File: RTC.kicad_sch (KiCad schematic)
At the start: 10 parts, among them U5 PCF8563TS, Y2 MC-306

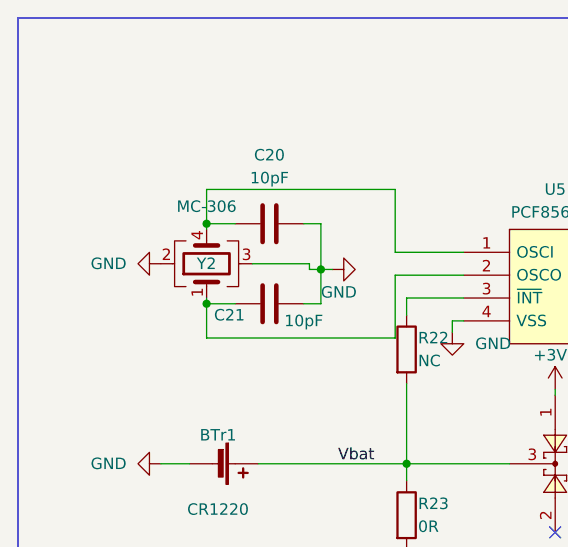
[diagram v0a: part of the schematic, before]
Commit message: Feat: Components's layout
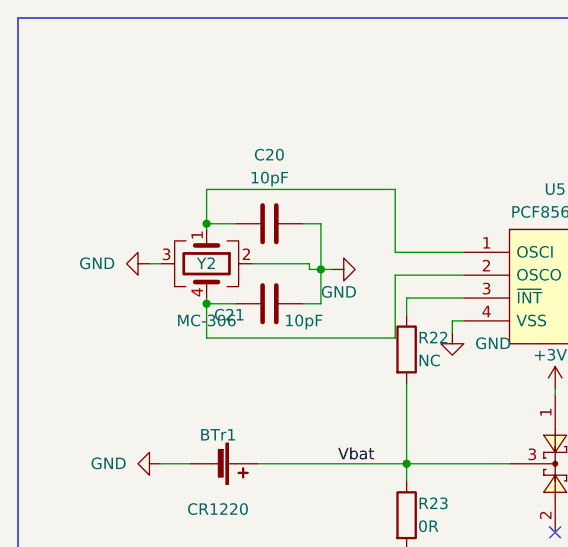
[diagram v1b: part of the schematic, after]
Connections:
- net at C21.1, U5.2 (OSCO): now also Y2.4; no longer Y2.1
- net at C20.1, U5.1 (OSCI): now also Y2.1; no longer Y2.4
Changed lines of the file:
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@@
+	(wire
+		(pts
+			(xy 51.435 51.435) (xy 52.705 51.435)
+		)
+		(stroke
+			(width 0)
+			(type default)
+		)
+	)
 	(wire
 		(pts
@@
 	(symbol
 		(lib_id "power:GND")
-		(at 52.705 51.435 270)
+		(at 51.435 51.435 270)
 		(unit 1)
 		(exclude_from_sim no)
@@
 		(fields_autoplaced yes)
 		(property "Reference" "#PWR031"
-			(at 46.355 51.435 0)
+			(at 45.085 51.435 0)
 			(effects
 				(font
@@
 		)
 		(property "Value" "GND"
-			(at 48.895 51.4349 90)
+			(at 47.625 51.4349 90)
 			(effects
 				(font
@@
 		)
 		(property "Footprint" ""
-			(at 52.705 51.435 0)
+			(at 51.435 51.435 0)
 			(effects
 				(font
@@
 		)
 		(property "Datasheet" ""
-			(at 52.705 51.435 0)
+			(at 51.435 51.435 0)
 			(effects
 				(font
@@
 		)
 		(property "Description" ""
-			(at 52.705 51.435 0)
+			(at 51.435 51.435 0)
 			(effects
 				(font
@@
 	)
 	(symbol
+		(lib_id "Device:Crystal_GND23")
+		(at 57.785 51.435 270)
+		(unit 1)
+		(exclude_from_sim no)
+		(in_bom yes)
+		(on_board yes)
+		(dnp no)
+		(property "Reference" "Y2"
+			(at 57.785 51.435 90)
+			(effects
+				(font
+					(size 1.27 1.27)
+				)
+			)
+		)
+		(property "Value" "MC-306"
+			(at 57.785 57.785 90)
+			(effects
+				(font
+					(size 1.27 1.27)
+				)
+			)
+		)
+		(property "Footprint" "Crystal:Crystal_SMD_SeikoEpson_MC306-4Pin_8.0x3.2mm"
+			(at 57.785 51.435 0)
+			(effects
+				(font
+					(size 1.27 1.27)
+				)
+				(hide yes)
+			)
+		)
+		(property "Datasheet" "~"
+			(at 57.785 51.435 0)
+			(effects
+				(font
+					(size 1.27 1.27)
+				)
+				(hide yes)
+			)
+		)
+		(property "Description" ""
+			(at 57.785 51.435 0)
+			(effects
+				(font
+					(size 1.27 1.27)
+				)
+				(hide yes)
+			)
+		)
+		(pin "1"
+		)
+		(pin "2"
+		)
+		(pin "3"
+		)
+		(pin "4"
+		)
+		(instances
+			(project "DongTamV2"
+				(path "/2303d546-b88a-4ab0-aee1-26e3b32ac9d7/4db09d46-189e-4d6b-adc1-7214f7292c64"
+					(reference "Y2")
+					(unit 1)
+				)
+			)
+		)
+	)
+	(symbol
 		(lib_id "Device:R")
 		(at 80.01 79.375 0)
@@
 					(unit 1)
 				)
-			)
-		)
-	)
-	(symbol
-		(lib_id "Device:Crystal_GND23")
-		(at 57.785 51.435 90)
-		(unit 1)
-		(exclude_from_sim no)
-		(in_bom yes)
-		(on_board yes)
-		(dnp no)
-		(property "Reference" "Y2"
-			(at 57.785 51.435 90)
-			(effects
-				(font
-					(size 1.27 1.27)
-				)
-			)
-		)
-		(property "Value" "MC-306"
-			(at 57.785 45.085 90)
-			(effects
-				(font
-					(size 1.27 1.27)
-				)
-			)
-		)
-		(property "Footprint" "Crystal:Crystal_SMD_SeikoEpson_MC306-4Pin_8.0x3.2mm"
-			(at 57.785 51.435 0)
-			(effects
-				(font
-					(size 1.27 1.27)
-				)
-				(hide yes)
-			)
-		)
-		(property "Datasheet" "~"
-			(at 57.785 51.435 0)
-			(effects
-				(font
-					(size 1.27 1.27)
-				)
-				(hide yes)
-			)
-		)
-		(property "Description" ""
-			(at 57.785 51.435 0)
-			(effects
-				(font
-					(size 1.27 1.27)
-				)
-				(hide yes)
-			)
-		)
-		(pin "1"
-		)
-		(pin "2"
-		)
-		(pin "3"
-		)
-		(pin "4"
-		)
-		(instances
-			(project "DongTamV2"
-				(path "/2303d546-b88a-4ab0-aee1-26e3b32ac9d7/4db09d46-189e-4d6b-adc1-7214f7292c64"
-					(reference "Y2")
-					(unit 1)
-				)
-			)
-			(project "dongtam"
-				(path "/6833aec4-3d1d-4261-9b3e-f0452b565dd3/a9a99304-d65b-4ed1-854e-7f464f20419d"
-					(reference "Y?")
-					(unit 1)
-				)

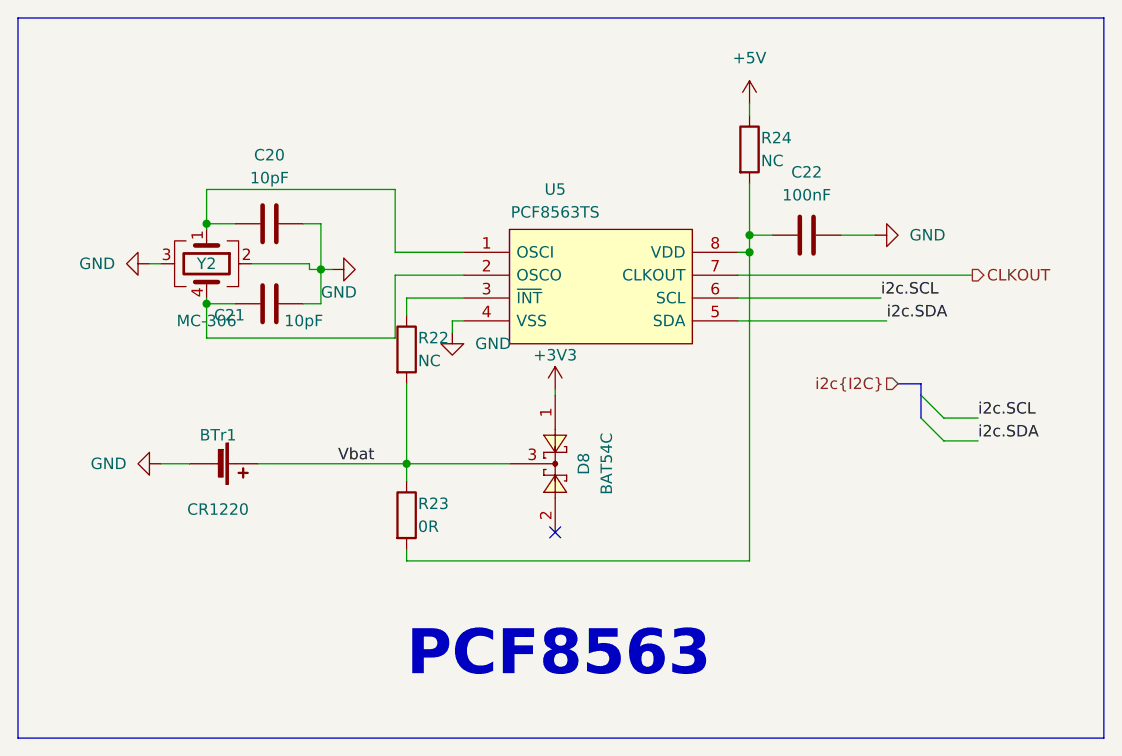
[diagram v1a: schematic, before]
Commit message: layout p1
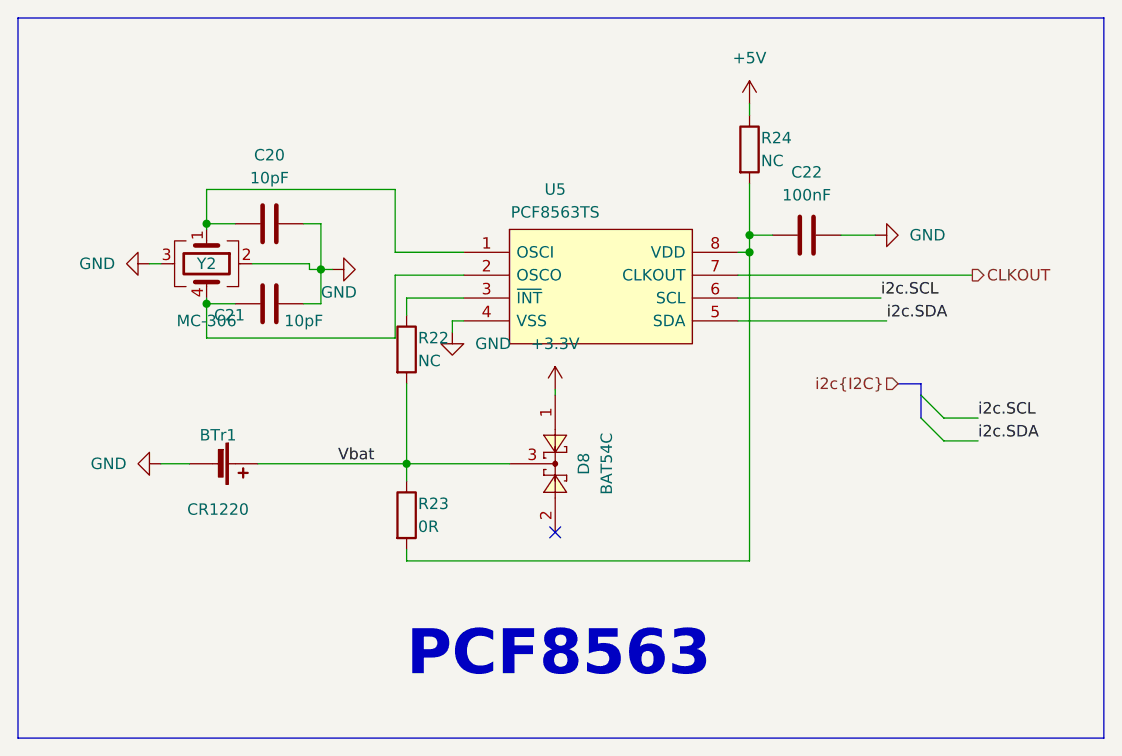
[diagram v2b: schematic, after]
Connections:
- net +3V3 renamed +3.3V
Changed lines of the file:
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@@
+	)
+	(symbol
+		(lib_id "power:+3.3V")
+		(at 96.52 65.405 0)
+		(unit 1)
+		(exclude_from_sim no)
+		(in_bom yes)
+		(on_board yes)
+		(dnp no)
+		(fields_autoplaced yes)
+		(property "Reference" "#PWR029"
+			(at 96.52 69.215 0)
+			(effects
+				(font
+					(size 1.27 1.27)
+				)
+				(hide yes)
+			)
+		)
+		(property "Value" "+3.3V"
+			(at 96.52 60.325 0)
+			(effects
+				(font
+					(size 1.27 1.27)
+				)
+			)
+		)
+		(property "Footprint" ""
+			(at 96.52 65.405 0)
+			(effects
+				(font
+					(size 1.27 1.27)
+				)
+				(hide yes)
+			)
+		)
+		(property "Datasheet" ""
+			(at 96.52 65.405 0)
+			(effects
+				(font
+					(size 1.27 1.27)
+				)
+				(hide yes)
+			)
+		)
+		(property "Description" "Power symbol creates a global label with name \"+3.3V\""
+			(at 96.52 65.405 0)
+			(effects
+				(font
+					(size 1.27 1.27)
+				)
+				(hide yes)
+			)
+		)
+		(pin "1"
+		)
+		(instances
+			(project "DongTamV2"
+				(path "/2303d546-b88a-4ab0-aee1-26e3b32ac9d7/4db09d46-189e-4d6b-adc1-7214f7292c64"
+					(reference "#PWR029")
+					(unit 1)
+				)
+			)
+		)
 	)
 	(symbol
@@
 					(unit 1)
 				)
-			)
-			(project "dongtam"
-				(path "/6833aec4-3d1d-4261-9b3e-f0452b565dd3/a9a99304-d65b-4ed1-854e-7f464f20419d"
-					(reference "#PWR?")
-					(unit 1)
-				)
-			)
-		)
-	)
-	(symbol
-		(lib_id "power:+3V3")
-		(at 96.52 65.405 0)
-		(unit 1)
-		(exclude_from_sim no)
-		(in_bom yes)
-		(on_board yes)
-		(dnp no)
-		(property "Reference" "#PWR035"
-			(at 96.52 69.215 0)
-			(effects
-				(font
-					(size 1.27 1.27)
-				)
-				(hide yes)
-			)
-		)
-		(property "Value" "+3V3"
-			(at 96.52 61.595 0)
-			(effects
-				(font
-					(size 1.27 1.27)
-				)
-			)
-		)
-		(property "Footprint" ""
-			(at 96.52 65.405 0)
-			(effects
-				(font
-					(size 1.27 1.27)
-				)
-				(hide yes)
-			)
-		)
-		(property "Datasheet" ""
-			(at 96.52 65.405 0)
-			(effects
-				(font
-					(size 1.27 1.27)
-				)
-				(hide yes)
-			)
-		)
-		(property "Description" ""
-			(at 96.52 65.405 0)
-			(effects
-				(font
-					(size 1.27 1.27)
-				)
-				(hide yes)
-			)
-		)
-		(pin "1"
-		)
-		(instances
-			(project "DongTamV2"
-				(path "/2303d546-b88a-4ab0-aee1-26e3b32ac9d7/4db09d46-189e-4d6b-adc1-7214f7292c64"
-					(reference "#PWR035")
-					(unit 1)
-				)
